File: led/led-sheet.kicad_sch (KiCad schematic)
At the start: 3 parts

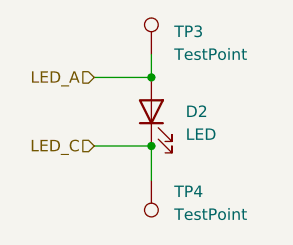
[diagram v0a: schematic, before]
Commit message: sch
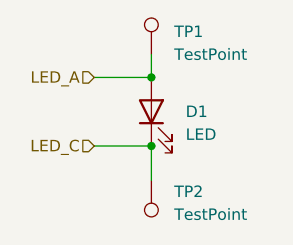
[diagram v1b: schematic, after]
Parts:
- renumbered D2 to D1, TP3 to TP1, TP4 to TP2
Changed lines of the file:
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@@
     (effects (font (size 1.27 1.27)) (justify right))
   )
-  (symbol (lib_id "Connector:TestPoint") (at 152.4 81.28 0)
+  (symbol (lib_id "Connector:TestPoint") (at 152.4 81.28 0) (unit 1)
     (in_bom yes) (on_board yes)
-    (property "Reference" "TP3" (id 0) (at 154.94 78.74 0)
+    (property "Reference" "TP1" (id 0) (at 154.94 78.74 0)
       (effects (font (size 1.27 1.27)) (justify left))
     )
@@
     )
   )
-  (symbol (lib_id "Connector:TestPoint") (at 152.4 95.25 180)
+  (symbol (lib_id "Connector:TestPoint") (at 152.4 95.25 180) (unit 1)
     (in_bom yes) (on_board yes)
-    (property "Reference" "TP4" (id 0) (at 154.94 96.52 0)
+    (property "Reference" "TP2" (id 0) (at 154.94 96.52 0)
       (effects (font (size 1.27 1.27)) (justify right))
     )
@@
     )
   )
-  (symbol (lib_id "Device:LED") (at 152.4 87.63 90)
+  (symbol (lib_id "Device:LED") (at 152.4 87.63 90) (unit 1)
     (in_bom yes) (on_board yes)
-    (property "Reference" "D2" (id 0) (at 156.21 87.63 90)
+    (property "Reference" "D1" (id 0) (at 156.21 87.63 90)
       (effects (font (size 1.27 1.27)) (justify right))
     )

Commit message: led
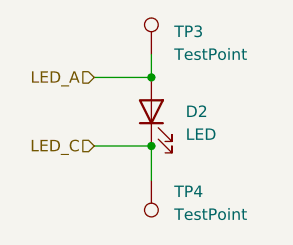
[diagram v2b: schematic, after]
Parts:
- renumbered D1 to D2, TP1 to TP3, TP2 to TP4
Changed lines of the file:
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@@
     (effects (font (size 1.27 1.27)) (justify right))
   )
-  (symbol (lib_id "Connector:TestPoint") (at 152.4 81.28 0) (unit 1)
+  (symbol (lib_id "Connector:TestPoint") (at 152.4 81.28 0)
     (in_bom yes) (on_board yes)
-    (property "Reference" "TP1" (id 0) (at 154.94 78.74 0)
+    (property "Reference" "TP3" (id 0) (at 154.94 78.74 0)
       (effects (font (size 1.27 1.27)) (justify left))
     )
@@
     )
   )
-  (symbol (lib_id "Connector:TestPoint") (at 152.4 95.25 180) (unit 1)
+  (symbol (lib_id "Connector:TestPoint") (at 152.4 95.25 180)
     (in_bom yes) (on_board yes)
-    (property "Reference" "TP2" (id 0) (at 154.94 96.52 0)
+    (property "Reference" "TP4" (id 0) (at 154.94 96.52 0)
       (effects (font (size 1.27 1.27)) (justify right))
     )
@@
     )
   )
-  (symbol (lib_id "Device:LED") (at 152.4 87.63 90) (unit 1)
+  (symbol (lib_id "Device:LED") (at 152.4 87.63 90)
     (in_bom yes) (on_board yes)
-    (property "Reference" "D1" (id 0) (at 156.21 87.63 90)
+    (property "Reference" "D2" (id 0) (at 156.21 87.63 90)
       (effects (font (size 1.27 1.27)) (justify right))
     )
